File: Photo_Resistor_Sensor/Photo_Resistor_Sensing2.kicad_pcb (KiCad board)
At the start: 2 copper layers, 108 x 62.2 mm, 20 parts, among them J1 Screw_Terminal_01x07, J2 Screw_Terminal_01x02

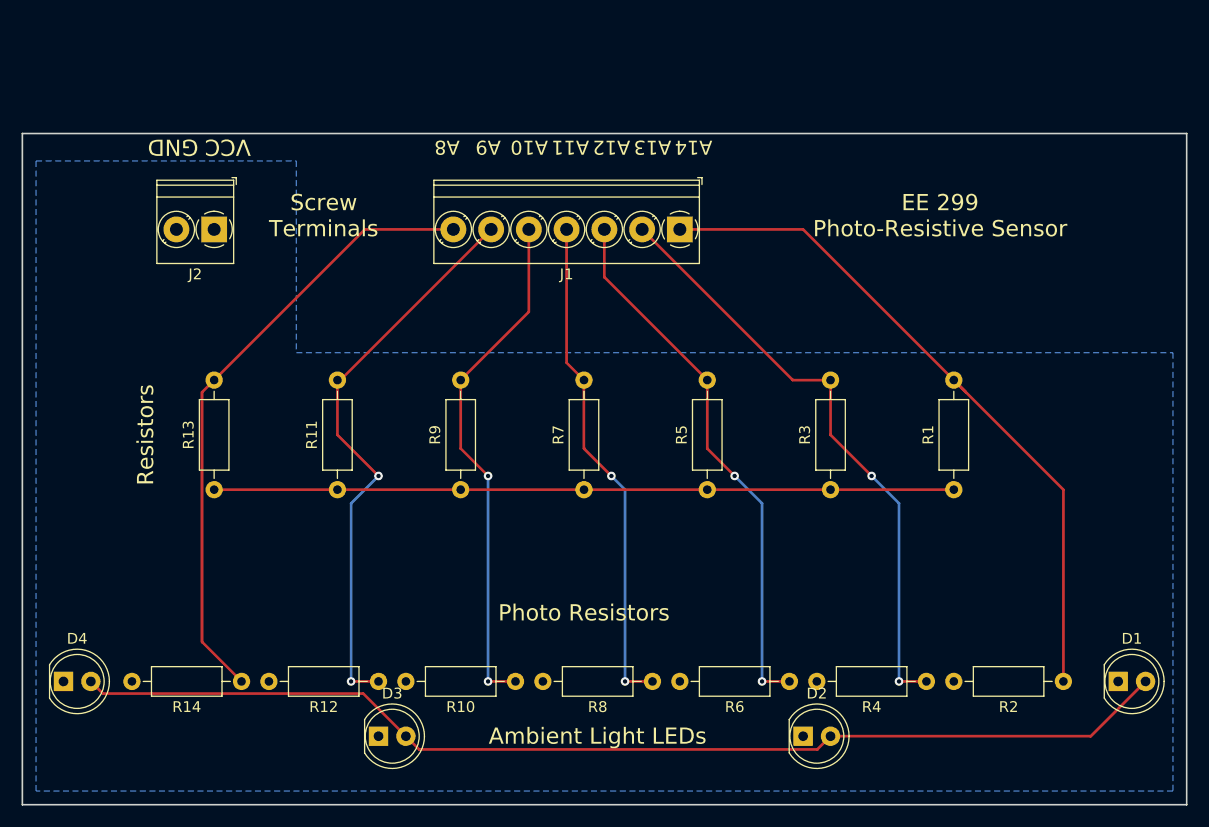
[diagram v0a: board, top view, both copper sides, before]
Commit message: I am a clown
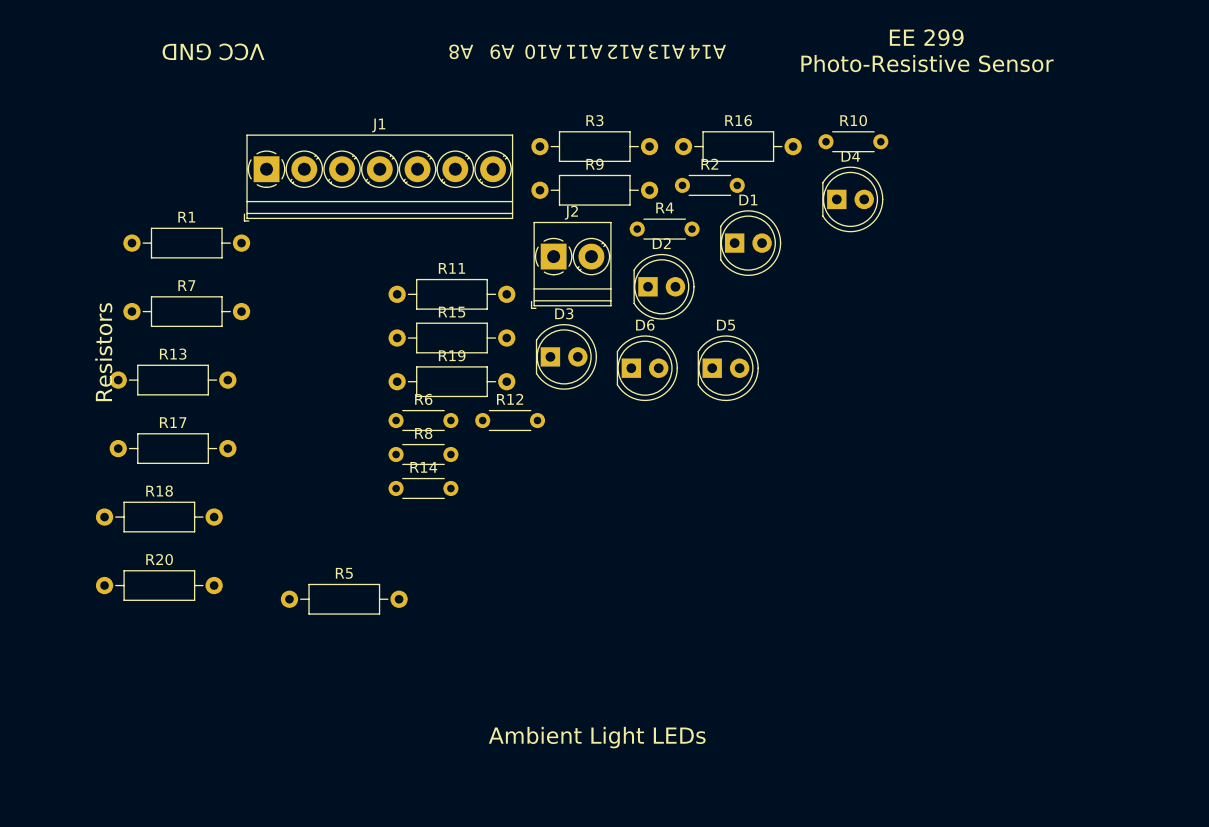
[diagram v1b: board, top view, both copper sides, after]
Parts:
- added D5: LED, LED_THT:LED_D5.0mm, F.Cu at (185.9, 77.6)
- added D6: LED, LED_THT:LED_D5.0mm, F.Cu at (178.4, 77.6)
- added R15: 330, Resistor_THT:R_Axial_DIN0207_L6.3mm_D2.5mm_P10.16mm_Horizontal, F.Cu at (156.7, 74.8)
- added R16: 330, Resistor_THT:R_Axial_DIN0207_L6.3mm_D2.5mm_P10.16mm_Horizontal, F.Cu at (183.2, 57.1)
- added R17: 330, Resistor_THT:R_Axial_DIN0207_L6.3mm_D2.5mm_P10.16mm_Horizontal, F.Cu at (130.8, 85.1)
- added R18: 330, Resistor_THT:R_Axial_DIN0207_L6.3mm_D2.5mm_P10.16mm_Horizontal, F.Cu at (129.5, 91.4)
- added R19: 330, Resistor_THT:R_Axial_DIN0207_L6.3mm_D2.5mm_P10.16mm_Horizontal, F.Cu at (156.7, 78.9)
- added R20: 330, Resistor_THT:R_Axial_DIN0207_L6.3mm_D2.5mm_P10.16mm_Horizontal, F.Cu at (129.5, 97.8)
- R1, R11, R13, R3, R5, R7, R9: value R -> 10k
- R10, R12, R14, R2, R4, R6, R8: footprint Resistor_THT:R_Axial_DIN0207_L6.3mm_D2.5mm_P10.16mm_Horizontal -> Resistor_THT:R_Axial_DIN0204_L3.6mm_D1.6mm_P5.08mm_Horizontal
- moved D4 84.5 mm to (197.4, 62.0)
- moved R1 79.6 mm to (132.1, 66.0), turned to 0 degrees
- moved R2 58.0 mm to (183.1, 60.7), turned to 0 degrees
- moved R10 57.7 mm to (196.4, 56.6), turned to 0 degrees
- moved D1 54.0 mm to (188.0, 66.0)
- moved R4 49.8 mm to (178.9, 64.7), turned to 0 degrees
- moved R7 45.0 mm to (132.1, 72.4), turned to 0 degrees
- moved D2 44.1 mm to (179.9, 70.1)
- moved R6 43.8 mm to (156.6, 82.5), turned to 0 degrees
- moved R3 41.7 mm to (169.9, 57.1), turned to 0 degrees
- moved R5 40.0 mm to (146.7, 99.1), turned to 0 degrees
- moved J1 38.7 mm to (144.6, 59.2), turned to 0 degrees
- moved D3 38.6 mm to (170.9, 76.6)
- moved R8 31.7 mm to (156.6, 85.6), turned to 0 degrees
- moved J2 31.6 mm to (171.2, 67.3), turned to 0 degrees
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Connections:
- D2 pad 2: Net-(D1-Pad2) -> Net-(D2-Pad2)
- D3 pad 2: Net-(D1-Pad2) -> Net-(D3-Pad2)
- D4 pad 2: Net-(D1-Pad2) -> Net-(D4-Pad2)
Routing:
- net Net-(D1-Pad2): track 103.0 -> 0.00 mm
- net Net-(R1-Pad1): track 68.6 -> 0.00 mm
- net /A8: track 64.9 -> 0.00 mm
- net /A14: track 57.9 -> 0.00 mm
- net /A9: track 56.4 -> 0.00 mm, vias 2 -> 0
- net /A13: track 53.1 -> 0.00 mm, vias 2 -> 0
- net /A10: track 50.5 -> 0.00 mm, vias 2 -> 0
- net /A12: track 48.1 -> 0.00 mm, vias 2 -> 0
- net /A11: track 46.7 -> 0.00 mm, vias 2 -> 0
- removed copper zone on B.Cu, net (none)
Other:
- board outline removed
- net class Default removed
- board text removed: "Photo Resistors"
- board text removed: "Screw Terminals"
